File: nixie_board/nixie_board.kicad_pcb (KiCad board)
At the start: 2 copper layers, 215.9 x 53.3 mm, 71 parts, among them J1 12V, J2 170V, J3 GND, J4 SHDN, M1 MountingHole_3.2mm_M3, M2 MountingHole_3.2mm_M3, M3 MountingHole_3.2mm_M3, M4 MountingHole_3.2mm_M3, U1 74LS32, U10 74LS32, U11 K155NA1, U12 L7805, U13 74HCT595, U14 K155NA1, U15 DS18B20, U2 K155NA1, U3 WeMos_D1_mini, U4 74HCT595, U5 K155NA1, U6 74LS32, U7 K155NA1, U8 74HCT595, U9 K155NA1

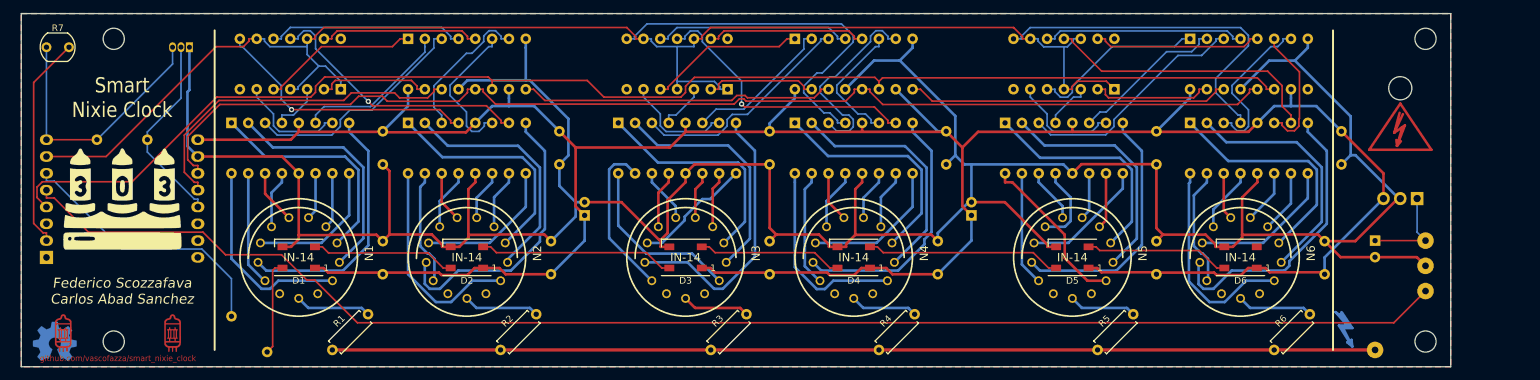
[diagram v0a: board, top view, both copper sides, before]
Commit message: final board review
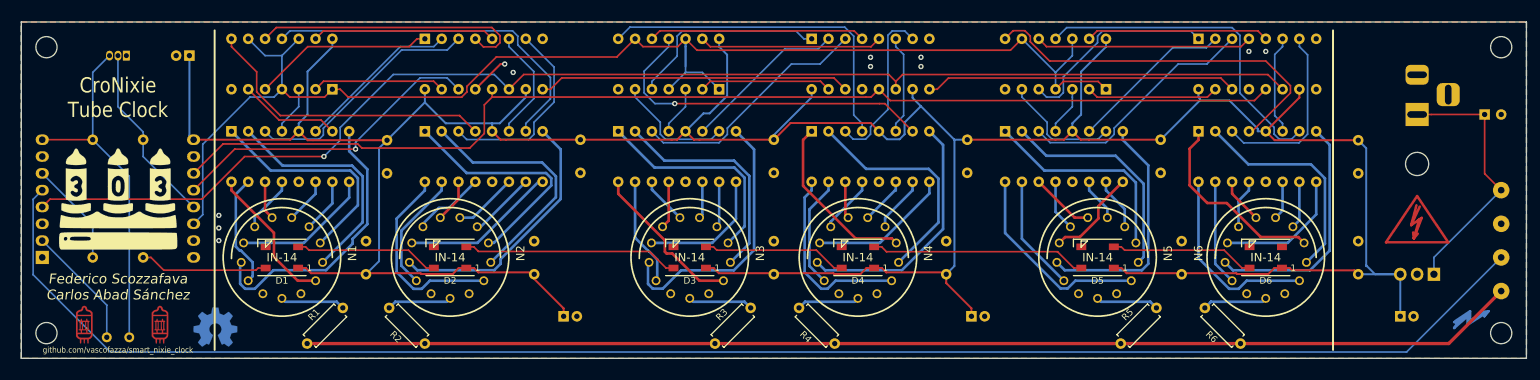
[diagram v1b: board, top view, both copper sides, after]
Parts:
- added C16: 10uF, Capacitor_THT:CP_Radial_D5.0mm_P2.00mm, B.Cu at (66.0, 26.7)
- added C17: 10uF, Capacitor_THT:CP_Radial_D5.0mm_P2.00mm, B.Cu at (248.9, 66.0)
- added J5: Barrel_Jack_Switch, Connector_BarrelJack:BarrelJack_Horizontal, B.Cu at (251.5, 35.6)
- R7: moved to B.Cu
- moved R7 45.6 mm to (57.0, 69.2), turned to 180 degrees
- moved C7 25.2 mm to (261.7, 35.6), turned to 0 degrees
- moved S3 24.4 mm to (70.0, 67.7)
- moved R8 22.8 mm to (51.4, 57.1), turned to 0 degrees
- moved J2 21.0 mm to (264.2, 62.2), turned to 270 degrees
- moved S1 19.1 mm to (260.2, 65.7), turned to 270 degrees
- moved C8 15.6 mm to (122.6, 66.0), turned to 0 degrees
- moved C15 15.2 mm to (184.2, 66.0), turned to 0 degrees
- moved S2 14.2 mm to (251.5, 52.1)
- moved J1 13.7 mm to (264.2, 47.0)
- moved J3 13.1 mm to (264.2, 52.1)
- moved J4 12.5 mm to (264.2, 57.1)
- moved U12 11.7 mm to (254.0, 59.7)
- moved M2 11.5 mm to (264.2, 25.4)
- moved M3 11.5 mm to (264.2, 68.6)
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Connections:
- U1 pad 14: (no net) -> /5V
- U1 pad 7: (no net) -> GND
- U10 pad 14: (no net) -> /5V
- U10 pad 7: (no net) -> GND
- U3 pad 14: Net-(U3-Pad14) -> /STROBE
- U3 pad 7: /STROBE -> Net-(U3-Pad7)
- U6 pad 14: (no net) -> /5V
- U6 pad 7: (no net) -> GND
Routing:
- net GND: track 467.4 -> 6.02 mm, vias 0 -> 11
- net /5V: track 411.9 -> 502.0 mm
- net /SHUTDOWN: track 219.2 -> 245.8 mm
- net /170V: track 157.5 -> 183.6 mm
- net Net-(C7-Pad1): track 14.5 -> 39.6 mm
- net /RGB: track 40.9 -> 15.9 mm
- net Net-(R7-Pad2): track 32.5 -> 18.6 mm
- net Net-(U1-Pad11): track 40.8 -> 54.4 mm, vias 1 -> 0
- net /3.3V: track 40.3 -> 53.5 mm
- net Net-(U1-Pad10): track 29.8 -> 42.3 mm
- net /STROBE: track 217.8 -> 206.0 mm
- net Net-(U6-Pad11): track 42.3 -> 52.7 mm
- net Net-(N1-Pad0): track 30.5 -> 21.8 mm
- net Net-(N4-Pad8): track 35.0 -> 26.4 mm
- net Net-(U10-Pad11): track 42.3 -> 50.7 mm
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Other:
- board size 215.9 x 53.3 mm -> 227.3 x 50.8 mm
- net class 5v rail: clearance 0.35 -> 0.254; trace_width 0.4 -> 0.3
- net class HighVoltageOut: clearance 0.35 -> 0.3
- board text added: "CroNixie Tube Clock"
- board text added: "Federico Scozzafava Carlos Abad Sánchez"
- board text added: "JLCJLCJLCJLC"
- board text removed: "Federico Scozzafava Carlos Abad Sanchez"
- board text removed: "Smart Nixie Clock"
